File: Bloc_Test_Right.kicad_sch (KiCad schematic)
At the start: 45 parts, among them Q29 2N7000, Q30 2N7000, Q31 2N7000, Q32 2N7000, Q33 2N7000, Q34 2N7000

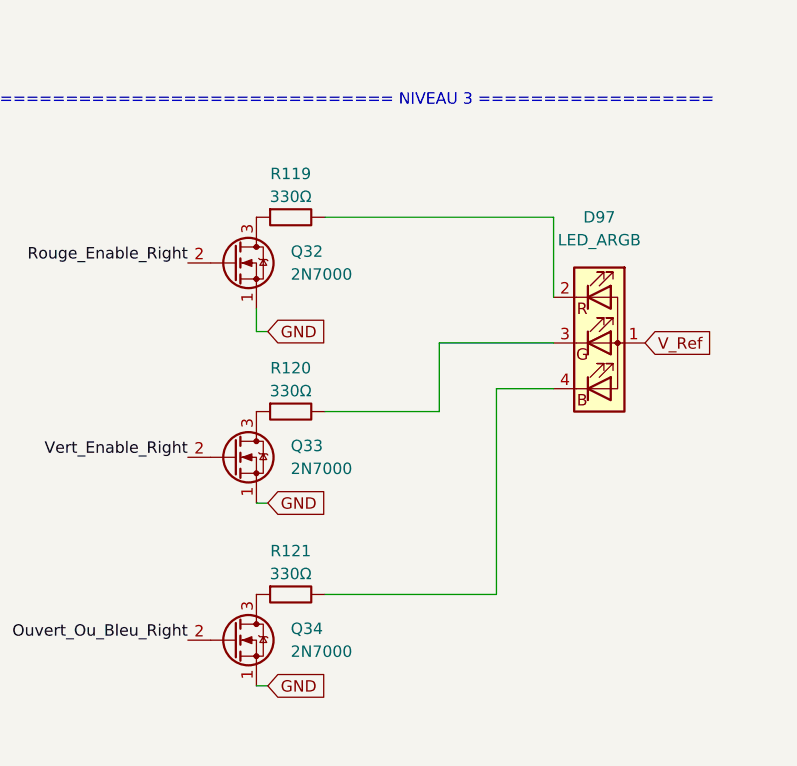
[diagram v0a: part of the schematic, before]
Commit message: Add files via upload
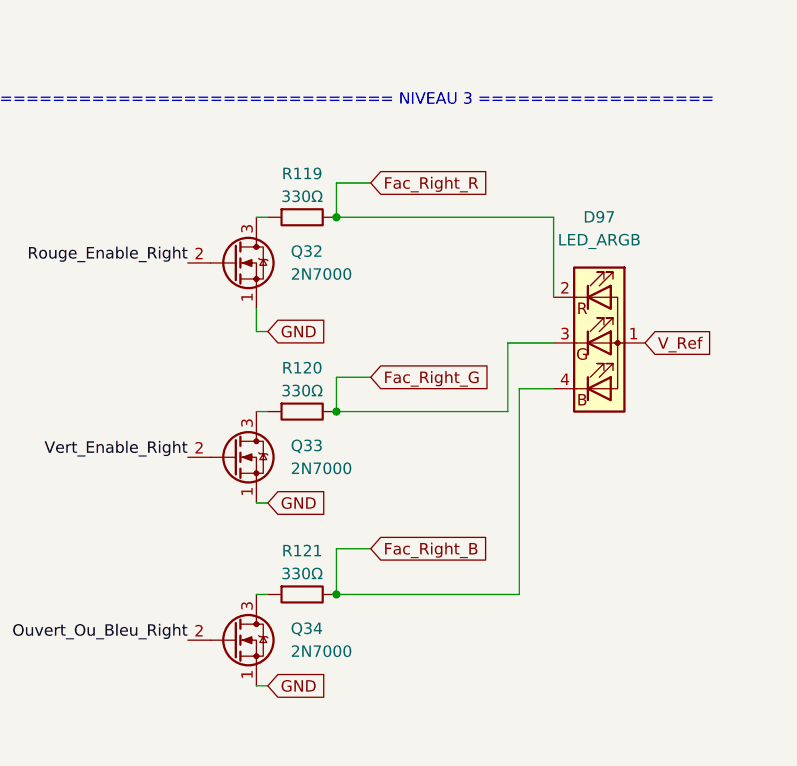
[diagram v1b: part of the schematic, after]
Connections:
- net Fac_Right_B: now reaches D97.4 (BK), R121.2
- net Fac_Right_R: now reaches D97.2 (RK), R119.2
- net Fac_Right_G: now reaches D97.3 (GK), R120.2
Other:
- moved on the sheet: R119, R120, R121
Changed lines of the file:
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@@
 	)
 	(junction
+		(at 240.03 121.92)
+		(diameter 0)
+		(color 0 0 0 0)
+	)
+	(junction
 		(at 148.59 58.42)
 		(diameter 0)
@@
 	)
 	(junction
+		(at 240.03 142.24)
+		(diameter 0)
+		(color 0 0 0 0)
+	)
+	(junction
 		(at 102.87 140.97)
 		(diameter 0)
@@
 	)
 	(junction
+		(at 240.03 100.33)
+		(diameter 0)
+		(color 0 0 0 0)
+	)
+	(junction
 		(at 157.48 152.4)
 		(diameter 0)
@@
 	(wire
 		(pts
+			(xy 240.03 142.24) (xy 260.35 142.24)
+		)
+		(stroke
+			(width 0)
+			(type default)
+		)
+	)
+	(wire
+		(pts
 			(xy 55.88 86.36) (xy 55.88 97.79)
 		)
@@
 	(wire
 		(pts
+			(xy 240.03 137.16) (xy 240.03 142.24)
+		)
+		(stroke
+			(width 0)
+			(type default)
+		)
+	)
+	(wire
+		(pts
 			(xy 106.68 34.29) (xy 106.68 45.72)
 		)
@@
 	(wire
 		(pts
+			(xy 243.84 118.11) (xy 240.03 118.11)
+		)
+		(stroke
+			(width 0)
+			(type default)
+		)
+	)
+	(wire
+		(pts
 			(xy 83.82 132.08) (xy 90.17 132.08)
 		)
@@
 	(wire
 		(pts
-			(xy 257.81 119.38) (xy 257.81 142.24)
+			(xy 260.35 119.38) (xy 260.35 142.24)
+		)
+		(stroke
+			(width 0)
+			(type default)
+		)
+	)
+	(wire
+		(pts
+			(xy 240.03 100.33) (xy 264.16 100.33)
 		)
 		(stroke
@@
 	(wire
 		(pts
-			(xy 238.76 142.24) (xy 257.81 142.24)
-		)
-		(stroke
-			(width 0)
-			(type default)
-		)
-	)
-	(wire
-		(pts
 			(xy 26.67 60.96) (xy 29.21 60.96)
 		)
@@
 	(wire
 		(pts
+			(xy 240.03 118.11) (xy 240.03 121.92)
+		)
+		(stroke
+			(width 0)
+			(type default)
+		)
+	)
+	(wire
+		(pts
 			(xy 35.56 53.34) (xy 39.37 53.34)
 		)
@@
 	(wire
 		(pts
-			(xy 238.76 100.33) (xy 264.16 100.33)
+			(xy 232.41 100.33) (xy 231.14 100.33)
 		)
 		(stroke
@@
 	(wire
 		(pts
-			(xy 251.46 114.3) (xy 251.46 121.92)
+			(xy 259.08 114.3) (xy 259.08 121.92)
 		)
 		(stroke
@@
 	(wire
 		(pts
+			(xy 243.84 96.52) (xy 240.03 96.52)
+		)
+		(stroke
+			(width 0)
+			(type default)
+		)
+	)
+	(wire
+		(pts
 			(xy 153.67 133.35) (xy 157.48 133.35)
 		)
@@
 	(wire
 		(pts
+			(xy 232.41 121.92) (xy 231.14 121.92)
+		)
+		(stroke
+			(width 0)
+			(type default)
+		)
+	)
+	(wire
+		(pts
 			(xy 90.17 156.21) (xy 102.87 156.21)
 		)
@@
 	(wire
 		(pts
-			(xy 257.81 119.38) (xy 264.16 119.38)
+			(xy 260.35 119.38) (xy 264.16 119.38)
+		)
+		(stroke
+			(width 0)
+			(type default)
+		)
+	)
+	(wire
+		(pts
+			(xy 259.08 114.3) (xy 264.16 114.3)
 		)
 		(stroke
@@
 	(wire
 		(pts
-			(xy 251.46 114.3) (xy 264.16 114.3)
+			(xy 240.03 121.92) (xy 259.08 121.92)
 		)
 		(stroke
@@
 	(wire
 		(pts
+			(xy 243.84 137.16) (xy 240.03 137.16)
+		)
+		(stroke
+			(width 0)
+			(type default)
+		)
+	)
+	(wire
+		(pts
 			(xy 264.16 100.33) (xy 264.16 109.22)
 		)
@@
 	(wire
 		(pts
-			(xy 238.76 121.92) (xy 251.46 121.92)
+			(xy 232.41 142.24) (xy 231.14 142.24)
+		)
+		(stroke
+			(width 0)
+			(type default)
+		)
+	)
+	(wire
+		(pts
+			(xy 240.03 96.52) (xy 240.03 100.33)
 		)
 		(stroke
@@
 		)
 	)
+	(global_label "Fac_Right_R"
+		(shape input)
+		(at 243.84 96.52 0)
+		(fields_autoplaced yes)
+		(effects
+			(font
+				(size 1.27 1.27)
+			)
+			(justify left)
+		)
+		(property "Intersheetrefs" "${INTERSHEET_REFS}"
+			(at 258.2551 96.52 0)
+			(hide yes)
+			(show_name no)
+			(do_not_autoplace no)
+			(effects
+				(font
+					(size 1.27 1.27)
+				)
+				(justify left)
+			)
+		)
+	)
 	(global_label "GND"
 		(shape input)
@@
 		)
 	)
+	(global_label "Fac_Right_G"
+		(shape input)
+		(at 243.84 118.11 0)
+		(fields_autoplaced yes)
+		(effects
+			(font
+				(size 1.27 1.27)
+			)
+			(justify left)
+		)
+		(property "Intersheetrefs" "${INTERSHEET_REFS}"
+			(at 258.2551 118.11 0)
+			(hide yes)
+			(show_name no)
+			(do_not_autoplace no)
+			(effects
+				(font
+					(size 1.27 1.27)
+				)
+				(justify left)
+			)
+		)
+	)
 	(global_label "Mode_Trailer"
 		(shape input)
@@
 		)
 	)
+	(global_label "Fac_Right_B"
+		(shape input)
+		(at 243.84 137.16 0)
+		(fields_autoplaced yes)
+		(effects
+			(font
+				(size 1.27 1.27)
+			)
+			(justify left)
+		)
+		(property "Intersheetrefs" "${INTERSHEET_REFS}"
+			(at 258.2551 137.16 0)
+			(hide yes)
+			(show_name no)
+			(do_not_autoplace no)
+			(effects
+				(font
+					(size 1.27 1.27)
+				)
+				(justify left)
+			)
+		)
+	)
 	(global_label "V_Ref"
 		(shape input)
@@
 	(symbol
 		(lib_id "PCM_SL_Resistors:330ohm")
-		(at 234.95 142.24 0)
+		(at 236.22 142.24 0)
 		(unit 1)
 		(body_style 1)
@@
 		(dnp no)
 		(property "Reference" "R121"
-			(at 234.95 137.414 0)
+			(at 236.22 137.414 0)
 			(show_name no)
 			(do_not_autoplace no)
@@
 		)
 		(property "Value" "330Ω"
-			(at 234.95 139.954 0)
+			(at 236.22 139.954 0)
 			(show_name no)
 			(do_not_autoplace no)
@@
 		)
 		(property "Footprint" "Resistor_THT:R_Axial_DIN0207_L6.3mm_D2.5mm_P10.16mm_Horizontal"
-			(at 235.839 146.558 0)
+			(at 237.109 146.558 0)
 			(hide yes)
 			(show_name no)
@@
 		)
 		(property "Datasheet" ""
-			(at 235.458 142.24 0)
+			(at 236.728 142.24 0)
 			(hide yes)
 			(show_name no)
@@
 		)
 		(property "Description" "330Ω, 1/4W Resistor"
-			(at 234.95 142.24 0)
+			(at 236.22 142.24 0)
 			(hide yes)
 			(show_name no)
@@
 	(symbol
 		(lib_id "PCM_SL_Resistors:330ohm")
-		(at 234.95 100.33 0)
+		(at 236.22 100.33 0)
 		(unit 1)
 		(body_style 1)
@@
 		(dnp no)
 		(property "Reference" "R119"
-			(at 234.95 95.504 0)
+			(at 236.22 95.504 0)
 			(show_name no)
 			(do_not_autoplace no)
@@
 		)
 		(property "Value" "330Ω"
-			(at 234.95 98.044 0)
+			(at 236.22 98.044 0)
 			(show_name no)
 			(do_not_autoplace no)
@@
 		)
 		(property "Footprint" "Resistor_THT:R_Axial_DIN0207_L6.3mm_D2.5mm_P10.16mm_Horizontal"
-			(at 235.839 104.648 0)
+			(at 237.109 104.648 0)
 			(hide yes)
 			(show_name no)
@@
 		)
 		(property "Datasheet" ""
-			(at 235.458 100.33 0)
+			(at 236.728 100.33 0)
 			(hide yes)
 			(show_name no)
@@
 		)
 		(property "Description" "330Ω, 1/4W Resistor"
-			(at 234.95 100.33 0)
+			(at 236.22 100.33 0)
 			(hide yes)
 			(show_name no)
@@
 	(symbol
 		(lib_id "PCM_SL_Resistors:330ohm")
-		(at 234.95 121.92 0)
+		(at 236.22 121.92 0)
 		(unit 1)
 		(body_style 1)
@@
 		(dnp no)
 		(property "Reference" "R120"
-			(at 234.95 117.094 0)
+			(at 236.22 117.094 0)
 			(show_name no)
 			(do_not_autoplace no)
@@
 		)
 		(property "Value" "330Ω"
-			(at 234.95 119.634 0)
+			(at 236.22 119.634 0)
 			(show_name no)
 			(do_not_autoplace no)
@@
 		)
 		(property "Footprint" "Resistor_THT:R_Axial_DIN0207_L6.3mm_D2.5mm_P10.16mm_Horizontal"
-			(at 235.839 126.238 0)
+			(at 237.109 126.238 0)
 			(hide yes)
 			(show_name no)
@@
 		)
 		(property "Datasheet" ""
-			(at 235.458 121.92 0)
+			(at 236.728 121.92 0)
 			(hide yes)
 			(show_name no)
@@
 		)
 		(property "Description" "330Ω, 1/4W Resistor"
-			(at 234.95 121.92 0)
+			(at 236.22 121.92 0)
 			(hide yes)
 			(show_name no)
